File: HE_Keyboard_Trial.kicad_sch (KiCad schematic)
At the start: 0 parts

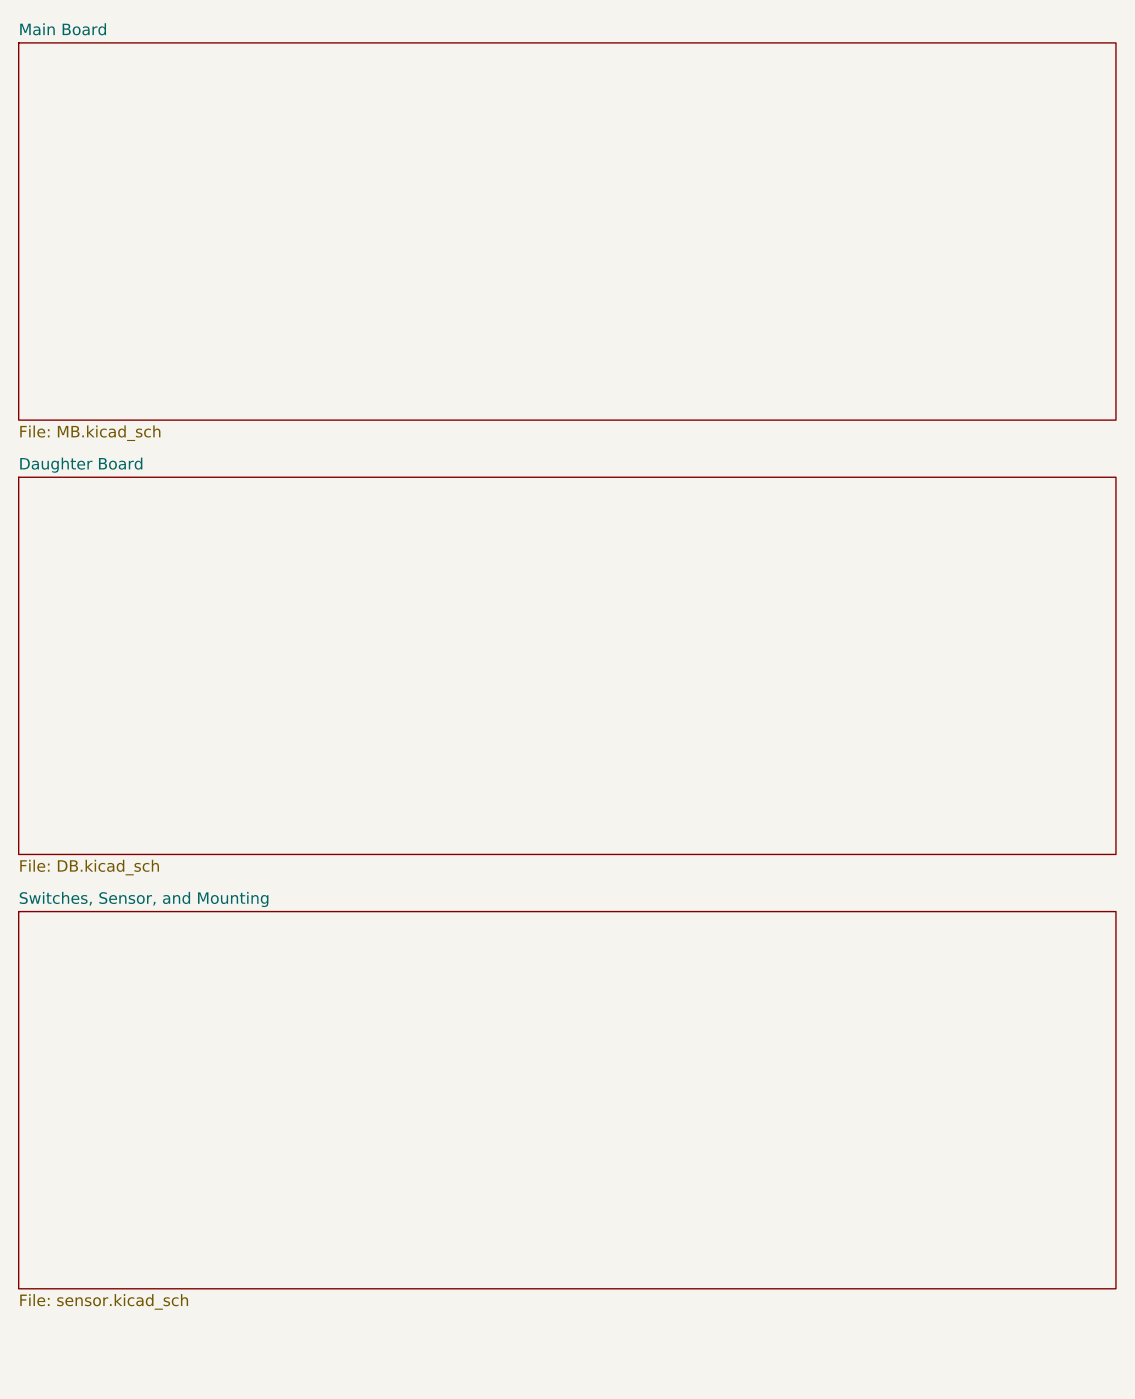
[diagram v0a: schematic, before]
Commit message: Fourth Commit
changing some name to not get sued :v
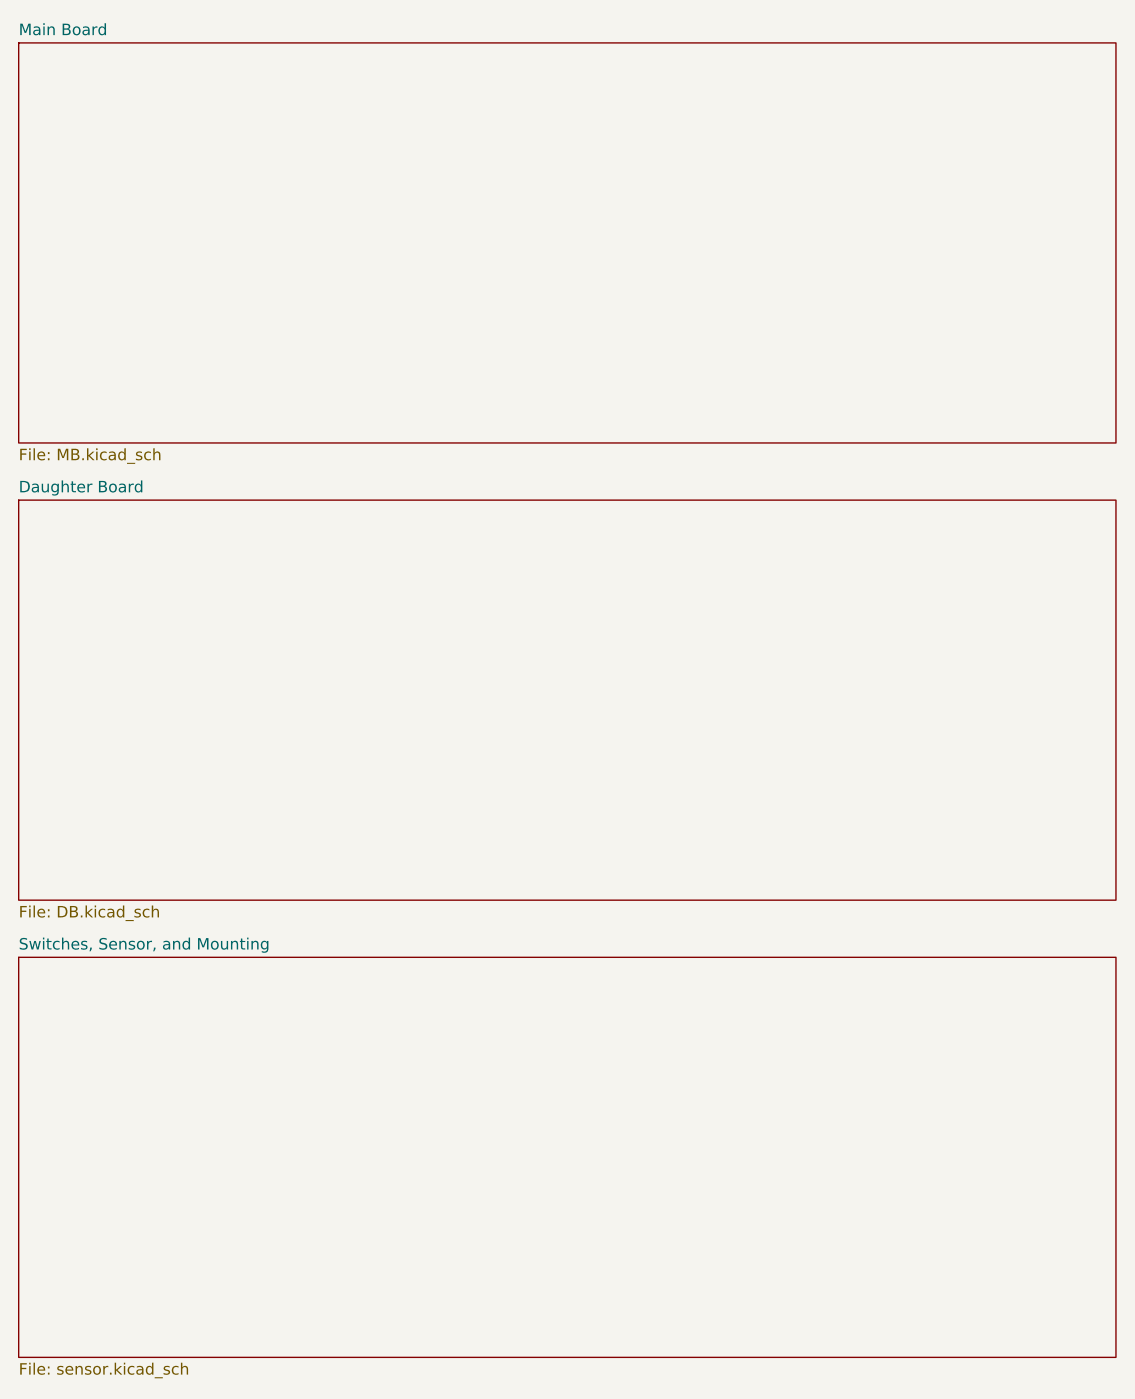
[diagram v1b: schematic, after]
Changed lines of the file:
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@@
 	)
 	(sheet
-		(at 12.7 111.76)
-		(size 121.92 41.91)
+		(at 12.7 116.84)
+		(size 121.92 44.45)
 		(fields_autoplaced yes)
 		(stroke
@@
 		)
 		(property "Sheetname" "Switches, Sensor, and Mounting"
-			(at 12.7 111.0484 0)
+			(at 12.7 116.1284 0)
 			(effects
 				(font
@@
 		)
 		(property "Sheetfile" "sensor.kicad_sch"
-			(at 12.7 154.2546 0)
+			(at 12.7 161.8746 0)
 			(effects
 				(font
@@
 	(sheet
 		(at 12.7 15.24)
-		(size 121.92 41.91)
+		(size 121.92 44.45)
 		(fields_autoplaced yes)
 		(stroke
@@
 		)
 		(property "Sheetfile" "MB.kicad_sch"
-			(at 12.7 57.7346 0)
+			(at 12.7 60.2746 0)
 			(effects
 				(font
@@
 	)
 	(sheet
-		(at 12.7 63.5)
-		(size 121.92 41.91)
+		(at 12.7 66.04)
+		(size 121.92 44.45)
 		(fields_autoplaced yes)
 		(stroke
@@
 		)
 		(property "Sheetname" "Daughter Board"
-			(at 12.7 62.7884 0)
+			(at 12.7 65.3284 0)
 			(effects
 				(font
@@
 		)
 		(property "Sheetfile" "DB.kicad_sch"
-			(at 12.7 105.9946 0)
+			(at 12.7 111.0746 0)
 			(effects
 				(font
